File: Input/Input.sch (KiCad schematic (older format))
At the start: 19 parts, among them J1 Conn_01x16, J2 Conn_01x16, J3 Conn_01x14, U1 74LS00, U2 74LS273, U3 74LS245

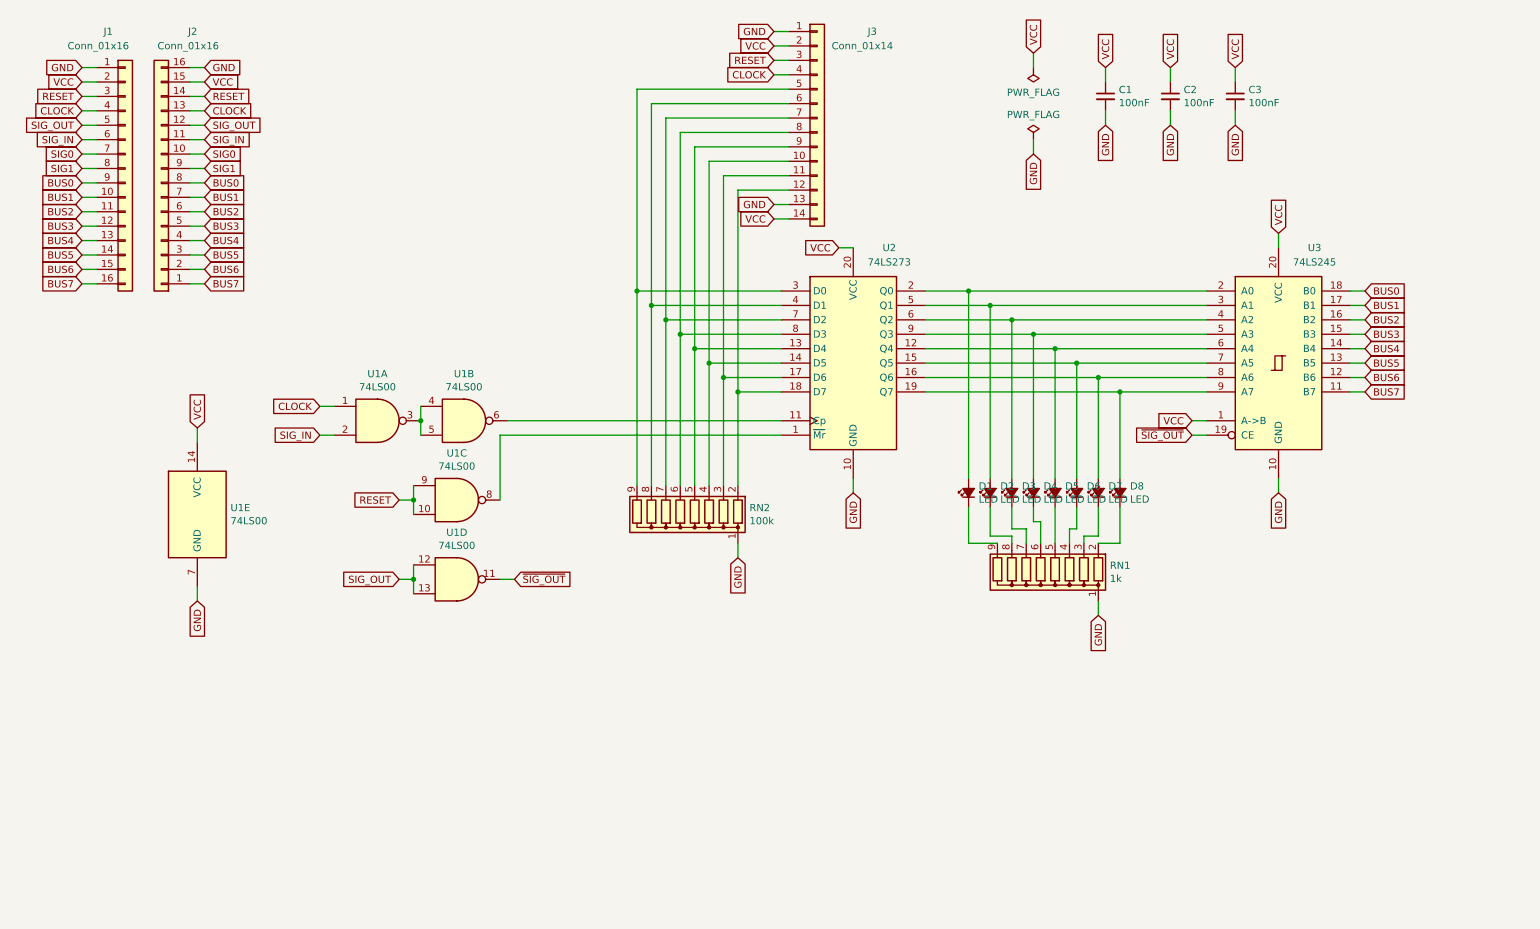
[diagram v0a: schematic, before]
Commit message: Update all boards to r3, and update revision log and gitignore
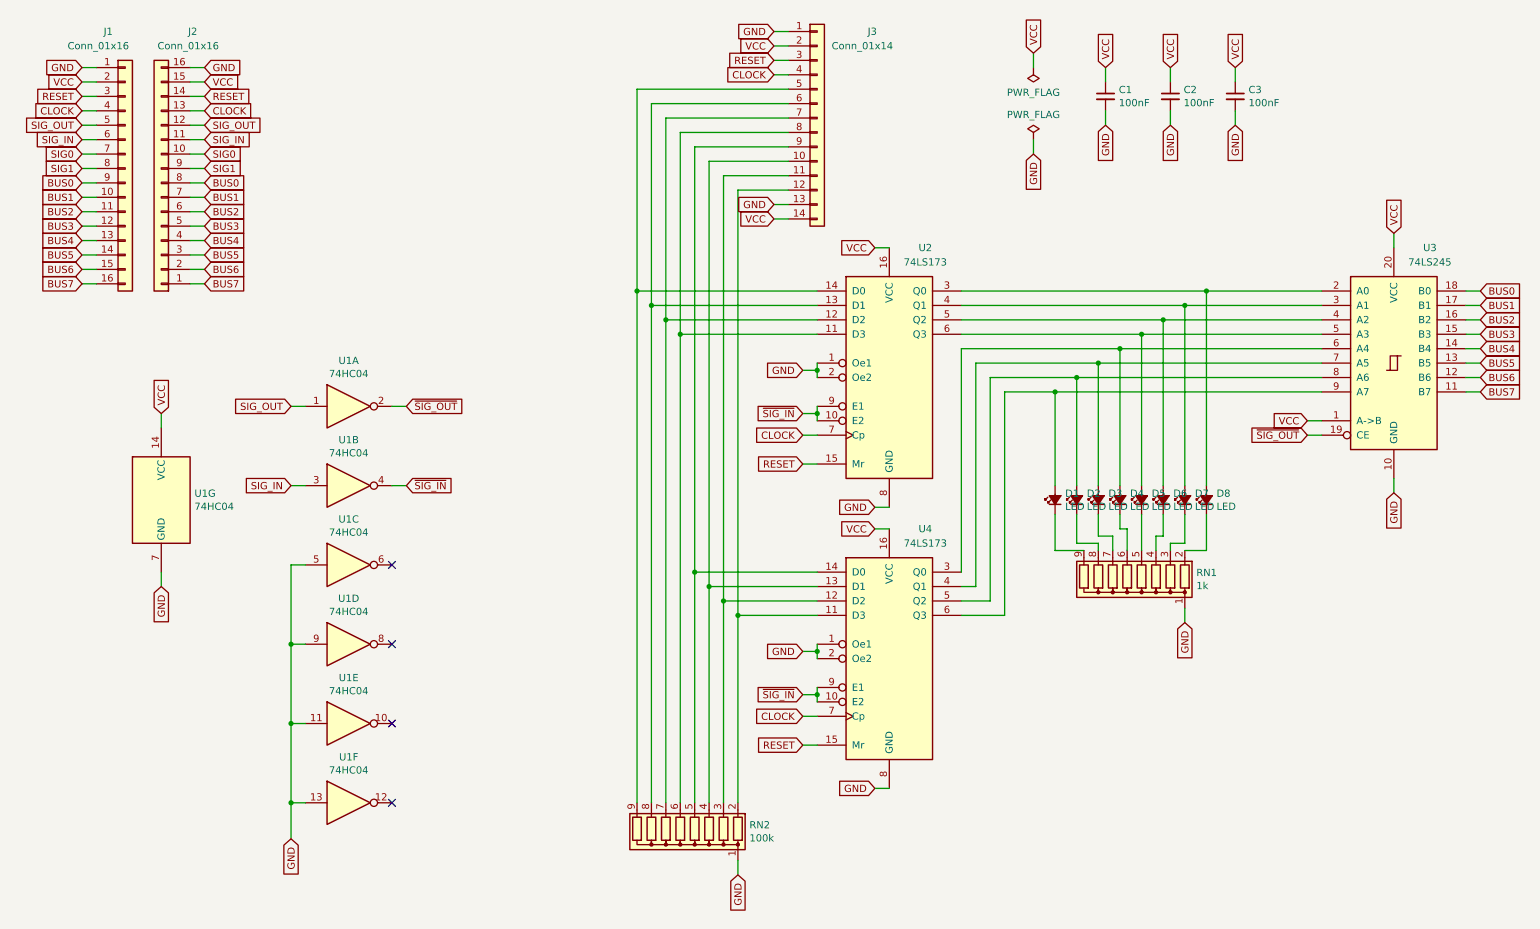
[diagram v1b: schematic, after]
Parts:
- removed U1: 74LS00, Package_DIP:DIP-14_W7.62mm, symbol 74xx:74LS00
- removed U2: 74LS273, Package_DIP:DIP-20_W7.62mm, symbol 74xx:74LS273
- added U1: 74HC04, symbol 74xx:74HC04
- added U2, U4: 74LS173, symbol 74xx:74LS173
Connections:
- net CLOCK: now also U2.7 (Cp), U4.7 (Cp)
- net GND: now also U1.11, U1.13, U1.5, U1.7 (GND), U1.9, U2.1 (Oe1), U2.2 (Oe2), U2.8 (GND), U4.1 (Oe1), U4.2 (Oe2), U4.8 (GND)
- net RESET: now also U2.15 (Mr), U4.15 (Mr)
- net SIG_IN: now also U1.3
- net SIG_OUT: now also U1.1
- net VCC: now also U1.14 (VCC), U2.16 (VCC), U4.16 (VCC)
- net ~SIG_OUT: now also U1.2
- net at U3.2 (A0): now also D8.2 (A), U2.3 (Q0); no longer D1.2 (A)
- net at U3.3 (A1): now also D7.2 (A), U2.4 (Q1); no longer D2.2 (A)
- net at U3.4 (A2): now also D6.2 (A), U2.5 (Q2); no longer D3.2 (A)
- net at U3.5 (A3): now also D5.2 (A), U2.6 (Q3); no longer D4.2 (A)
- net at U3.6 (A4): now also D4.2 (A), U4.3 (Q0); no longer D5.2 (A)
- net at U3.7 (A5): now also D3.2 (A), U4.4 (Q1); no longer D6.2 (A)
- net at U3.8 (A6): now also D2.2 (A), U4.5 (Q2); no longer D7.2 (A)
- net at U3.9 (A7): now also D1.2 (A), U4.6 (Q3); no longer D8.2 (A)
- net at J3.9 (Pin_9), RN2.5 (R4): now also U4.14 (D0)
- net at J3.10 (Pin_10), RN2.4 (R3): now also U4.13 (D1)
- net at J3.11 (Pin_11), RN2.3 (R2): now also U4.12 (D2)
- net at J3.12 (Pin_12), RN2.2 (R1): now also U4.11 (D3)
- net at J3.5 (Pin_5), RN2.9 (R8): now also U2.14 (D0)
- net at J3.6 (Pin_6), RN2.8 (R7): now also U2.13 (D1)
- net at J3.7 (Pin_7), RN2.7 (R6): now also U2.12 (D2)
- net at J3.8 (Pin_8), RN2.6 (R5): now also U2.11 (D3)
- new net ~SIG_IN: U1.4, U2.10 (E2), U2.9 (E1), U4.10 (E2), U4.9 (E1)
- no-connect marks 0 -> 4
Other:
- moved on the sheet: D1, D2, D3, D4, D5, D6, D7, D8, RN1, RN2, U3
